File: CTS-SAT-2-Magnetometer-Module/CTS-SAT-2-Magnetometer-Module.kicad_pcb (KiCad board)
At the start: 6 copper layers, 34.4 x 29.6 mm, 31 parts, among them J1 Conn_01x04_Pin, J2 SWD, SW1 SW_Push, U1 MMC5983MA, U2 LIS2MDL, U3 STM32F072C8Tx, U5 MIC5365-3.0YC5

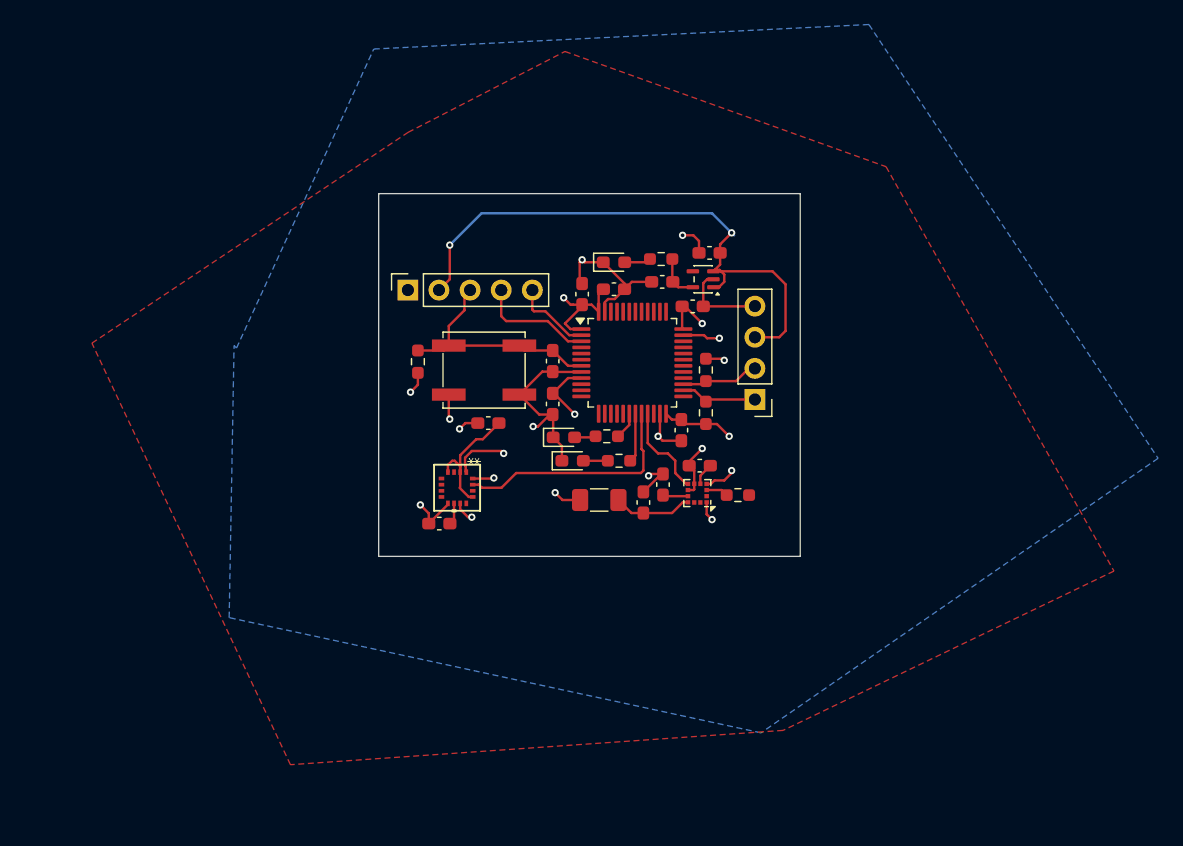
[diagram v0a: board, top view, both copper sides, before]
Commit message: Finished routing
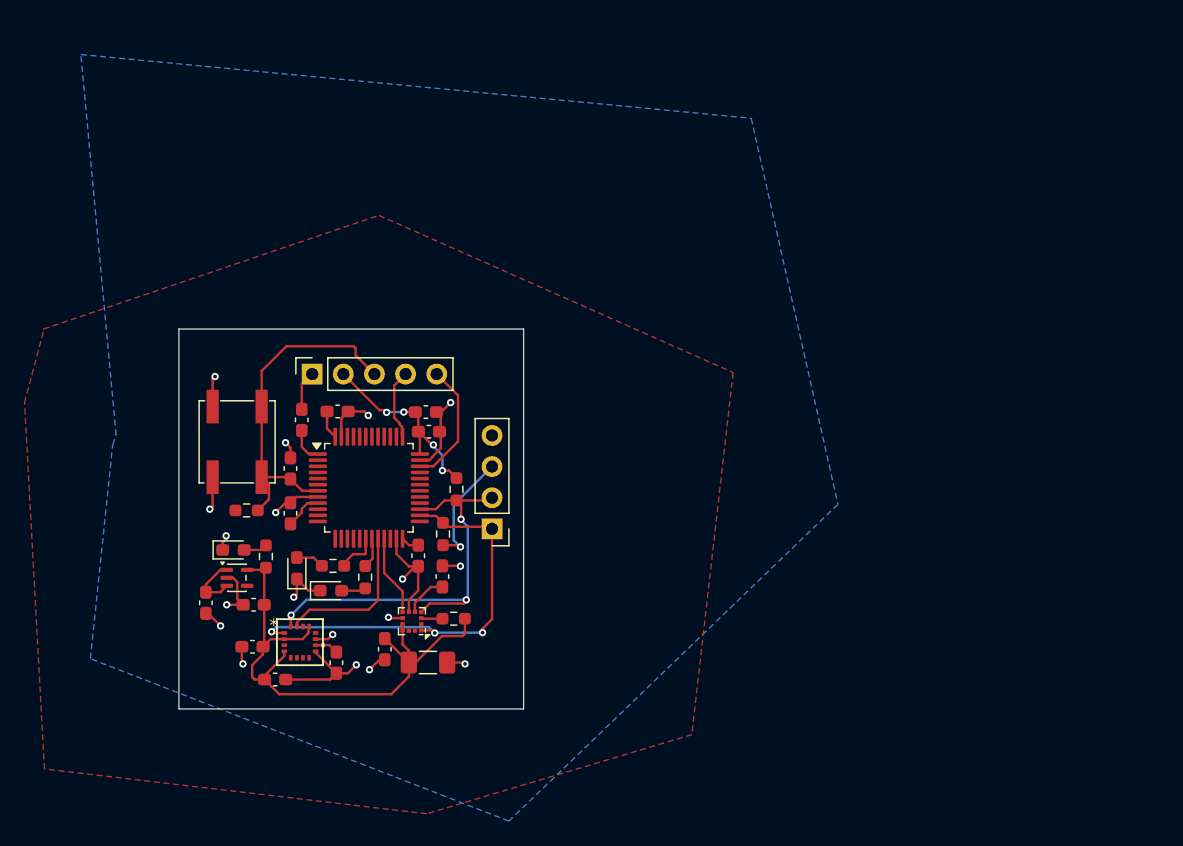
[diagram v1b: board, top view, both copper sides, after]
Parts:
- added C15: 10uF, Capacitor_SMD:C_0603_1608Metric_Pad1.08x0.95mm_HandSolder, F.Cu at (92.0, 174.8)
- C13: value 1uF1 -> 1uF
- C14: value 10uF1 -> 10uF
- C8: value 100nF1 -> 100nF
- moved C5 50.0 mm to (74.7, 178.6), turned to -90 degrees
- moved U5 45.2 mm to (77.2, 176.6), turned to 0 degrees
- moved C6 42.5 mm to (78.6, 178.8)
- moved R2 40.4 mm to (79.6, 174.8), turned to 90 degrees
- moved D2 38.9 mm to (77.0, 174.3)
- moved C9 36.9 mm to (81.6, 171.3), turned to -90 degrees
- moved C1 35.4 mm to (80.3, 184.8), turned to 180 degrees
- moved C10 31.0 mm to (82.5, 163.7), turned to 90 degrees
- moved C13 26.5 mm to (78.5, 182.2)
- moved U2 25.5 mm to (91.5, 180.1)
- moved R1 25.3 mm to (94.9, 179.9)
- moved R7 24.7 mm to (85.1, 175.6)
- moved D4 24.3 mm to (82.1, 175.8), turned to 90 degrees
- moved C4 24.3 mm to (89.3, 182.4), turned to -90 degrees
- moved J1 23.9 mm to (98.0, 172.6)
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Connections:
- C5 pad 1: Vdd -> +3V3
- J1 pad 3: Vdd -> +3V3
- J2 pad 2: Vdd -> +3V3
- U3 pad 2: SWCLK -> unconnected-(U3-PC13-Pad2)
- U3 pad 3: SWDIO -> unconnected-(U3-PC14-Pad3)
- U3 pad 34: unconnected-(U3-PA13-Pad34) -> SWCLK
- U3 pad 37: unconnected-(U3-PA14-Pad37) -> SWDIO
- U5 pad 1: Vdd -> +3V3
- U5 pad 3: Vdd -> +3V3
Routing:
- net Vdd: track 48.9 -> 0.00 mm, vias 2 -> 0
- net SDA: track 10.2 -> 34.7 mm, vias 2 -> 3
- net +3V0: track 23.0 -> 46.9 mm
- net SCL: track 12.1 -> 34.3 mm, vias 2 -> 3
- net +3V3: track 27.6 -> 41.0 mm, vias 6 -> 5
- net NRST: track 19.6 -> 28.4 mm
- net INT: track 19.3 -> 12.7 mm
- net SWDIO: track 9.52 -> 5.77 mm
- net SWCLK: track 6.46 -> 10.2 mm
- net Net-(U2-C1): track 1.81 -> 4.06 mm
- net Net-(U3-PB1): track 4.01 -> 1.99 mm
- net Net-(U3-PB0): track 2.22 -> 3.51 mm
- net DRDY: track 7.64 -> 6.60 mm
- net Net-(D4-A): track 1.75 -> 2.32 mm
- net GND: track 63.7 -> 63.3 mm, vias 12 -> 18
- added copper zone on F.Cu, net +3V3
- removed copper zone on F.Cu, net +3V0
- removed copper zone on In1.Cu, net +3V3
- removed copper zone on In2.Cu, net SCL
- removed copper zone on In4.Cu, net SDA
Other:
- board size 34.4 x 29.6 mm -> 28.1 x 31 mm
- copper layers 6 -> 2
